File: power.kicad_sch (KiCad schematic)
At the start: 0 parts

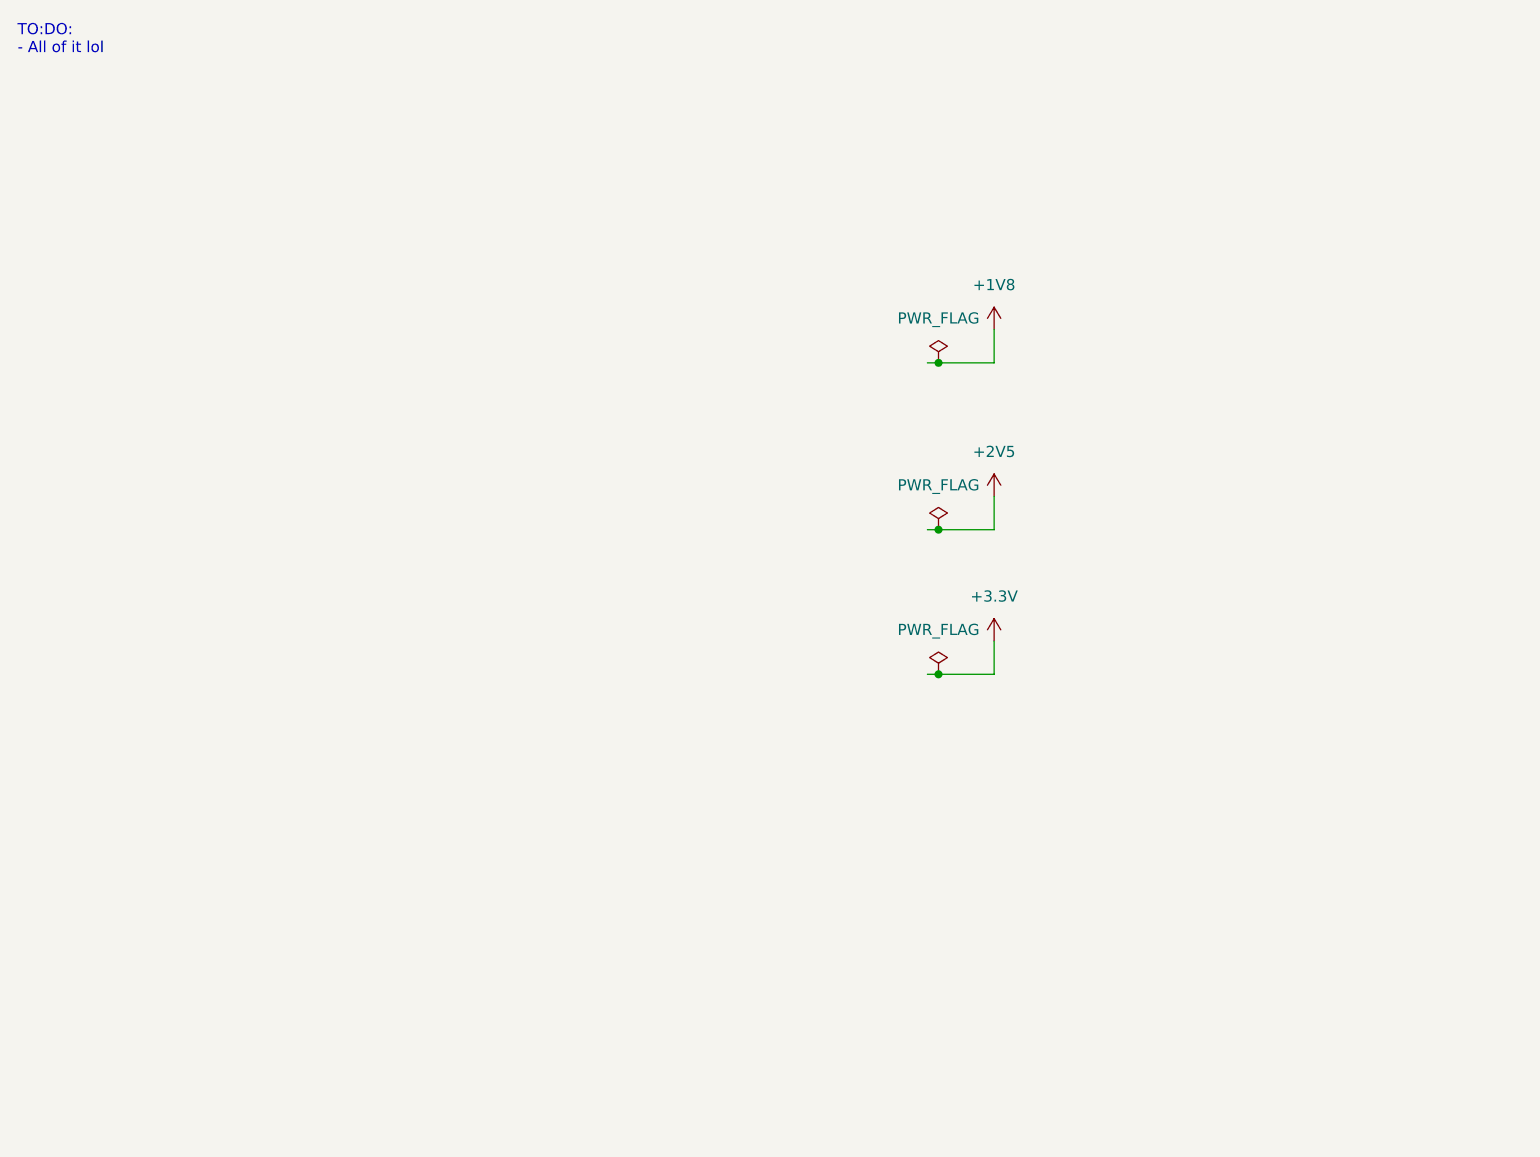
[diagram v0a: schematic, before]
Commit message: schematic capture like half done, need to do a lot of the smaller things
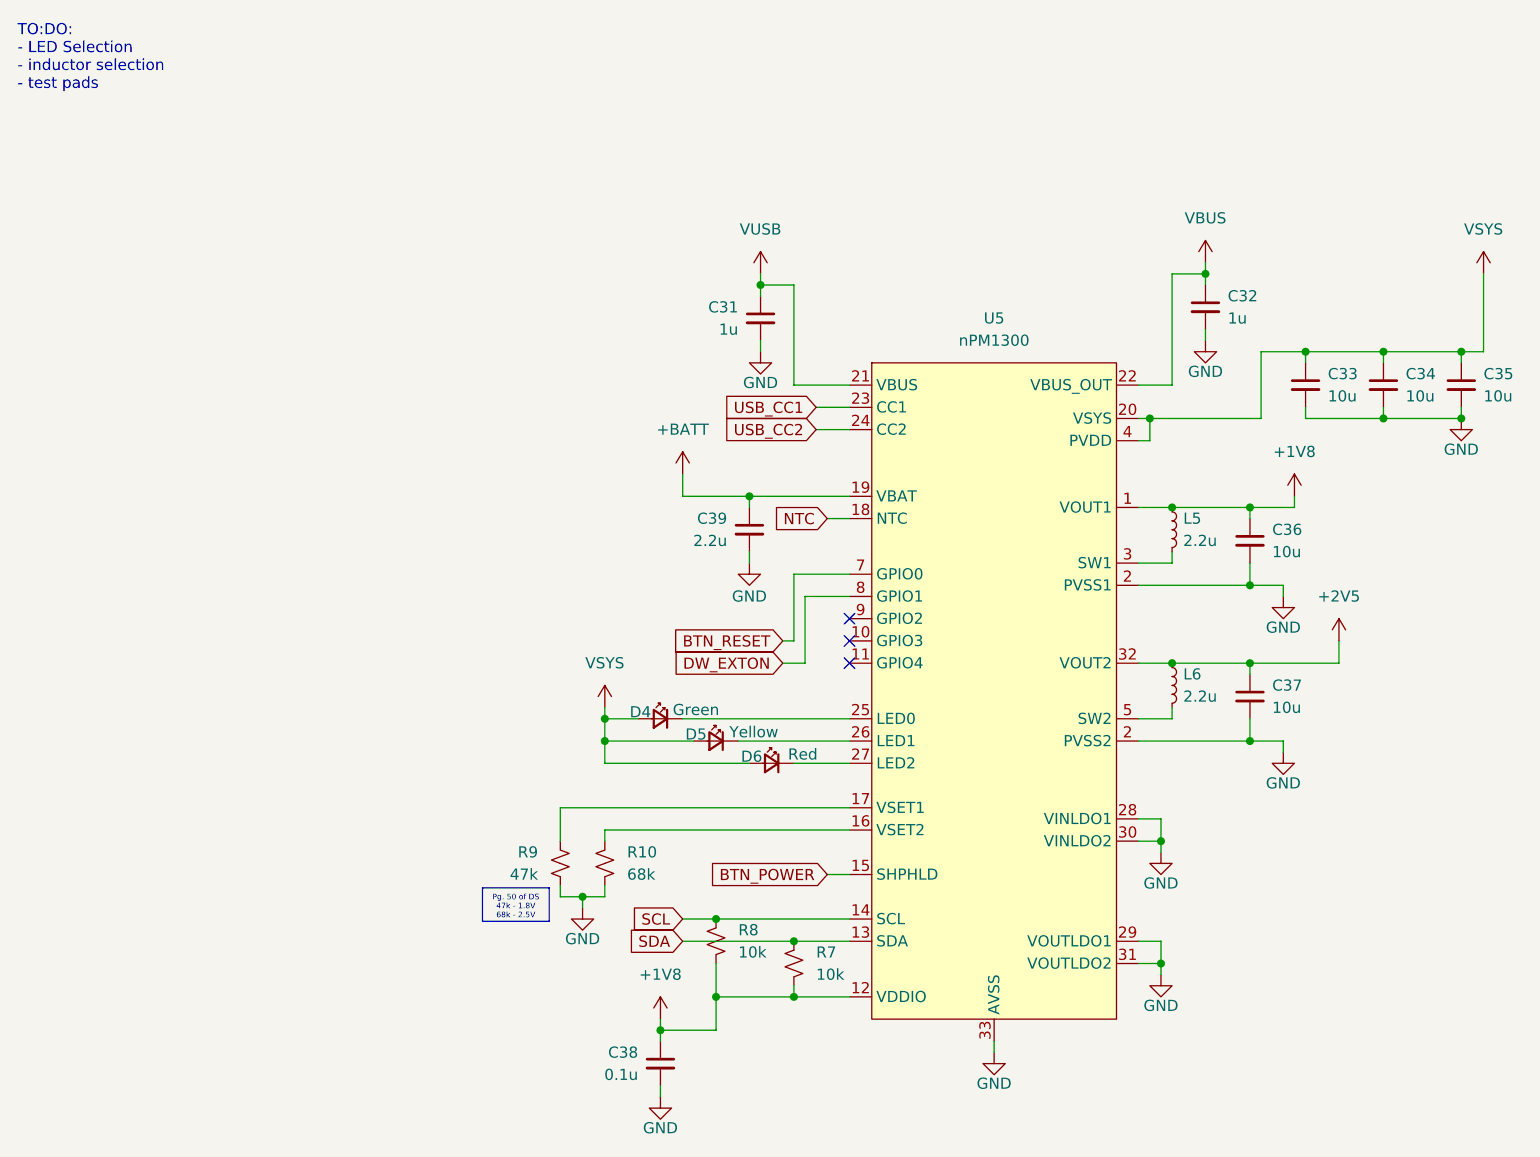
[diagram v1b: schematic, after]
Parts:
- added C31, C32: 1u, symbol Device:C_Small
- added C33, C34, C35, C36, C37: 10u, symbol Device:C_Small
- added C38: 0.1u, symbol Device:C_Small
- added C39: 2.2u, symbol Device:C_Small
- added D4: Green, symbol Device:LED_Small
- added D5: Yellow, symbol Device:LED_Small
- added D6: Red, symbol Device:LED_Small
- added L5, L6: 2.2u, symbol Device:L_Small
- added R10: 68k, symbol Device:R_Small_US
- added R7, R8: 10k, symbol Device:R_Small_US
- added R9: 47k, symbol Device:R_Small_US
- added U5: nPM1300, Package_DFN_QFN:QFN-40-1EP_5x5mm_P0.4mm_EP3.6x3.6mm_ThermalVias, symbol TrActor:nPM1300
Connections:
- net +1V8: now also C36.1, C38.1, L5.1, R7.2, R8.2, U5.1 (VOUT1), U5.12 (VDDIO)
- net +2V5: now also C37.1, L6.1, U5.32 (VOUT2)
- new net: R10.1, U5.16 (VSET2)
- new net: R9.1, U5.17 (VSET1)
- new net: D4.1 (K), U5.25 (LED0)
- new net: D5.1 (K), U5.26 (LED1)
- new net: D6.1 (K), U5.27 (LED2)
- new net: L5.2, U5.3 (SW1)
- new net: L6.2, U5.5 (SW2)
- new net +BATT: C39.1, U5.19 (VBAT)
- new net BTN_POWER: U5.15 (SHPHLD)
- new net BTN_RESET: U5.7 (GPIO0)
- new net DW_EXTON: U5.8 (GPIO1)
- new net GND: C31.2, C32.2, C33.2, C34.2, C35.2, C36.2, C37.2, C38.2, C39.2, R10.2, R9.2, U5.2 (PVSS2), U5.28 (VINLDO1), U5.29 (VOUTLDO1), U5.30 (VINLDO2), U5.31 (VOUTLDO2), U5.33 (AVSS)
- new net NTC: U5.18 (NTC)
- new net SCL: R8.1, U5.14 (SCL)
- new net SDA: R7.1, U5.13 (SDA)
- new net USB_CC1: U5.23 (CC1)
- new net USB_CC2: U5.24 (CC2)
- new net VBUS: C32.1, U5.22 (VBUS_OUT)
- new net VSYS: C33.1, C34.1, C35.1, D4.2 (A), D5.2 (A), D6.2 (A), U5.20 (VSYS), U5.4 (PVDD)
- new net VUSB: C31.1, U5.21 (VBUS)
- no-connect marks 0 -> 3
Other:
- note added: "Pg. 50 of DS 47k - 1.8V 68k - 2.5V"
- note added: "TO:DO: - LED Selection - inductor selection - test pads"
- note removed: "TO:DO: - All of it lol"
